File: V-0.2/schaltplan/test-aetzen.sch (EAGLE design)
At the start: 53 parts, among them IC1 MEGA32-A, IC2 NE5532N, Q1 BUZ21, X1 BU-SMB-H, X2 PN61729-S

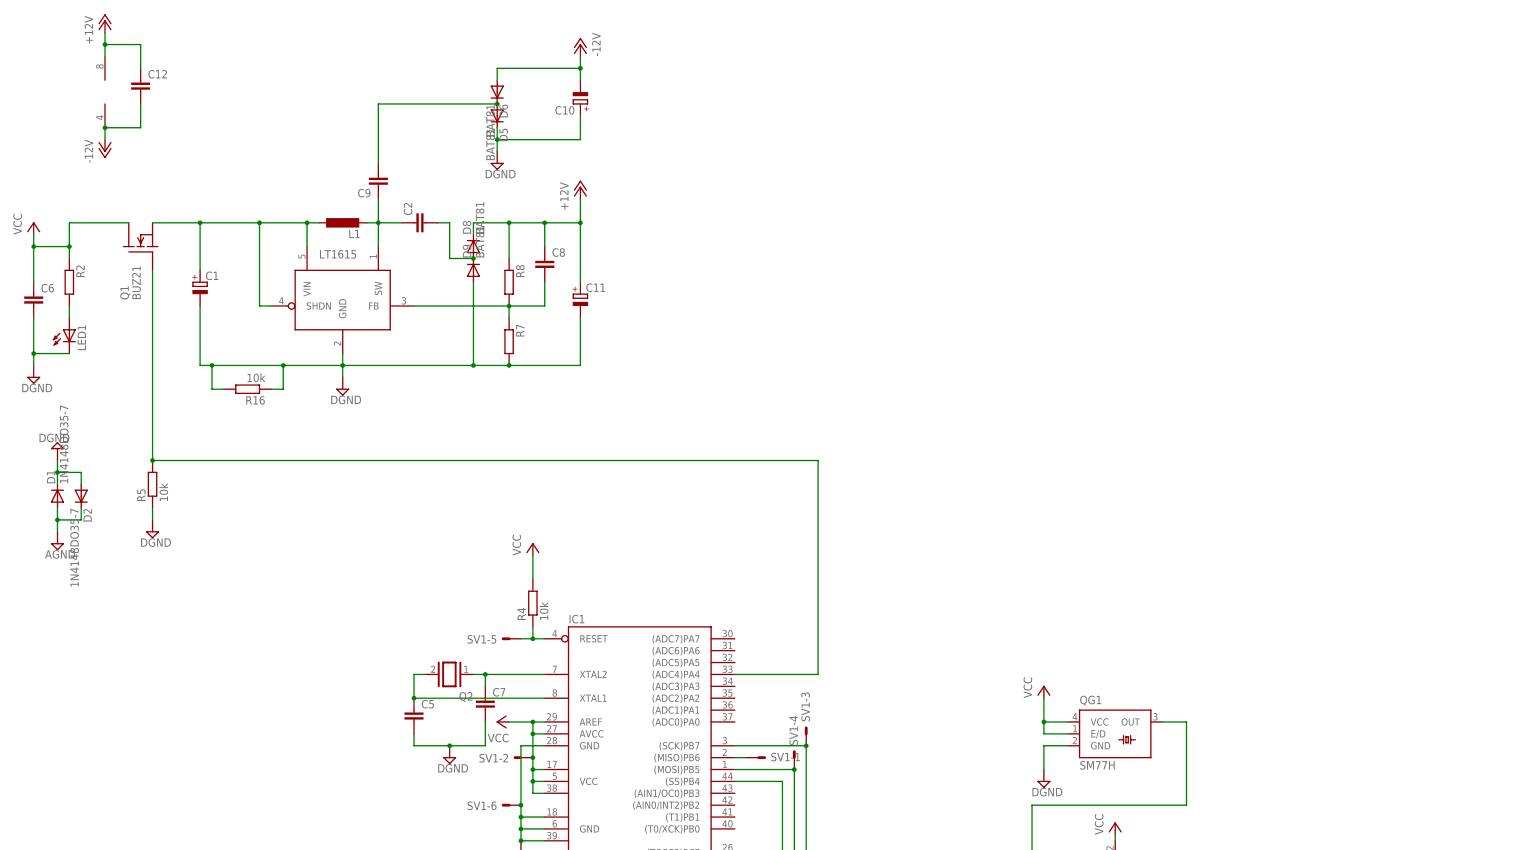
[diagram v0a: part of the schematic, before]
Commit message: another circuit diagramm for testing purposes
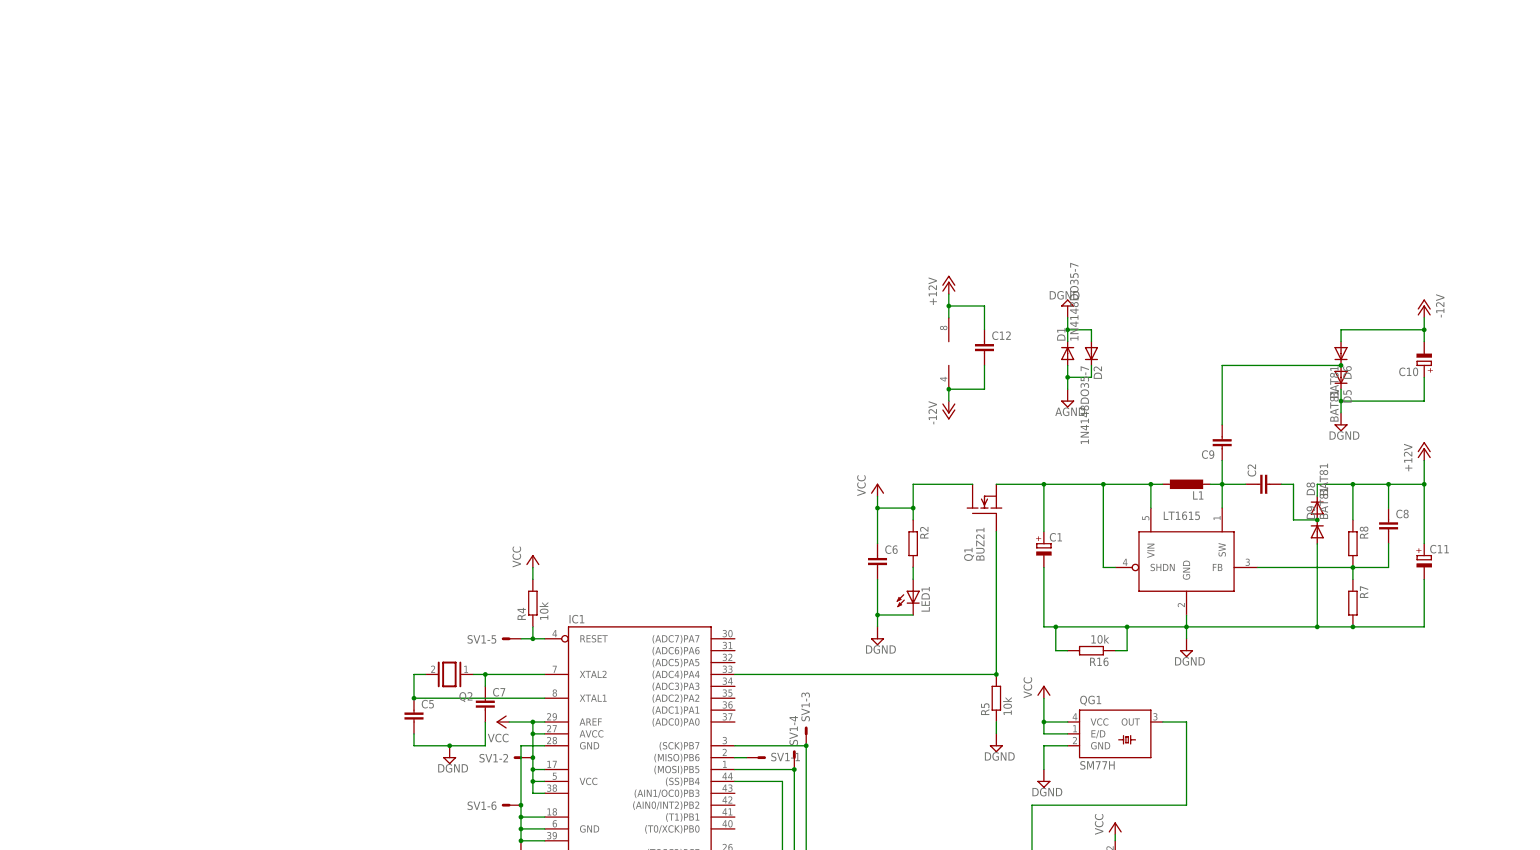
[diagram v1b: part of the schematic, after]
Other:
- moved on the sheet: C1, C10, C11, C12, C2, C6, C8, C9, D1, D2, D5, D6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
